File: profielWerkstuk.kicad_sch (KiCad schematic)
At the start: 94 parts, among them Q1 2N5179, SW1 SW_HF/VHF, SW2 SW_ANT, SW3 SW_PRESELECT_HFa, SW4 SW_PRESELECT_VHFa, SW5 SW_PRESELECT_HFb, SW6 SW_PRESELECT_VHFb, SW7 SW_SP5T_NR01105, T1 Transformer_1P_SS, T2 Transformer_1P_SS

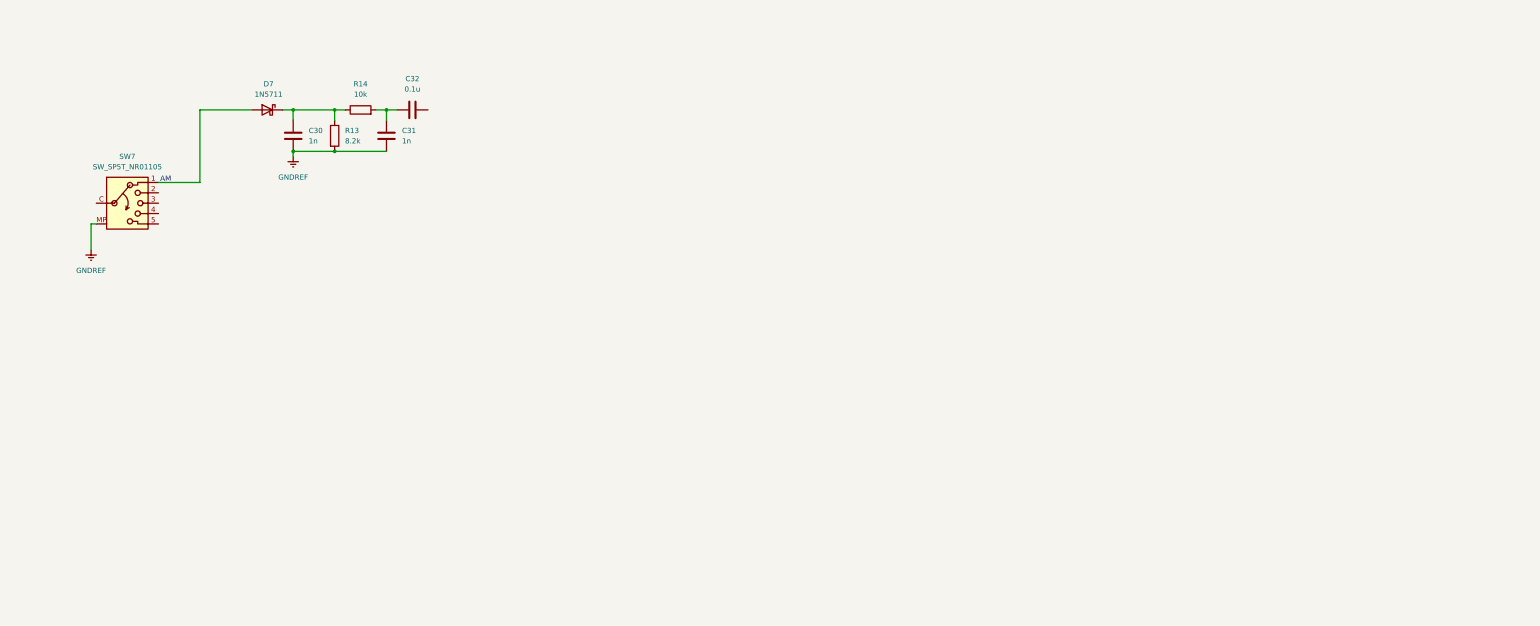
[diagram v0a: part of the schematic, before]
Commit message: did some organization
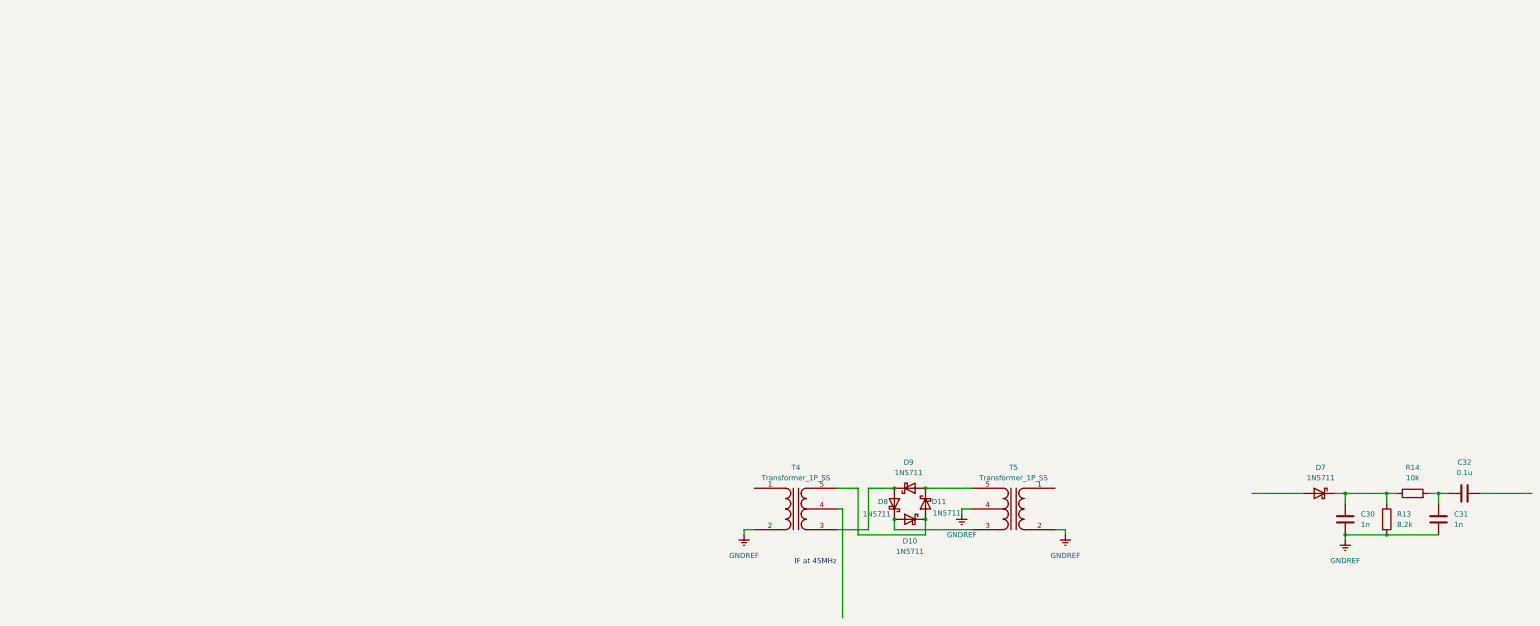
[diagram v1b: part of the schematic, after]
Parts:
- removed SW7: SW_SP5T_NR01105, Button_Switch_THT:SW_NKK_NR01, symbol Switch:SW_SP5T_NR01105
- added D10, D11, D8, D9: 1N5711, Diode_THT:D_DO-35_SOD27_P7.62mm_Horizontal, symbol Diode:1N5711
- added T4, T5: Transformer_1P_SS, symbol Device:Transformer_1P_SS
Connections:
- net GNDREF: now also T4.2 (AB), T5.2 (AB), T5.4 (SC)
- new net: D8.2 (A), D9.1 (K), T4.3 (SA)
- new net: D11.1 (K), D9.2 (A), T5.5 (SB)
- new net: D10.1 (K), D11.2 (A), T4.5 (SB)
- new net: D10.2 (A), D8.1 (K), T5.3 (SA)
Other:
- note removed: "AM"
- moved on the sheet: C30, C31, C32, D7, R13, R14
